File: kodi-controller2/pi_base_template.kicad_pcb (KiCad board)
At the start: 2 copper layers, 109.2 x 62.9 mm, 17 parts, among them P1 Raspberry_Pi_+_Conn, SW1 SW_PUSH_SMALL, SW2 SW_PUSH_SMALL, SW3 SW_PUSH_SMALL, SW4 SW_PUSH_SMALL

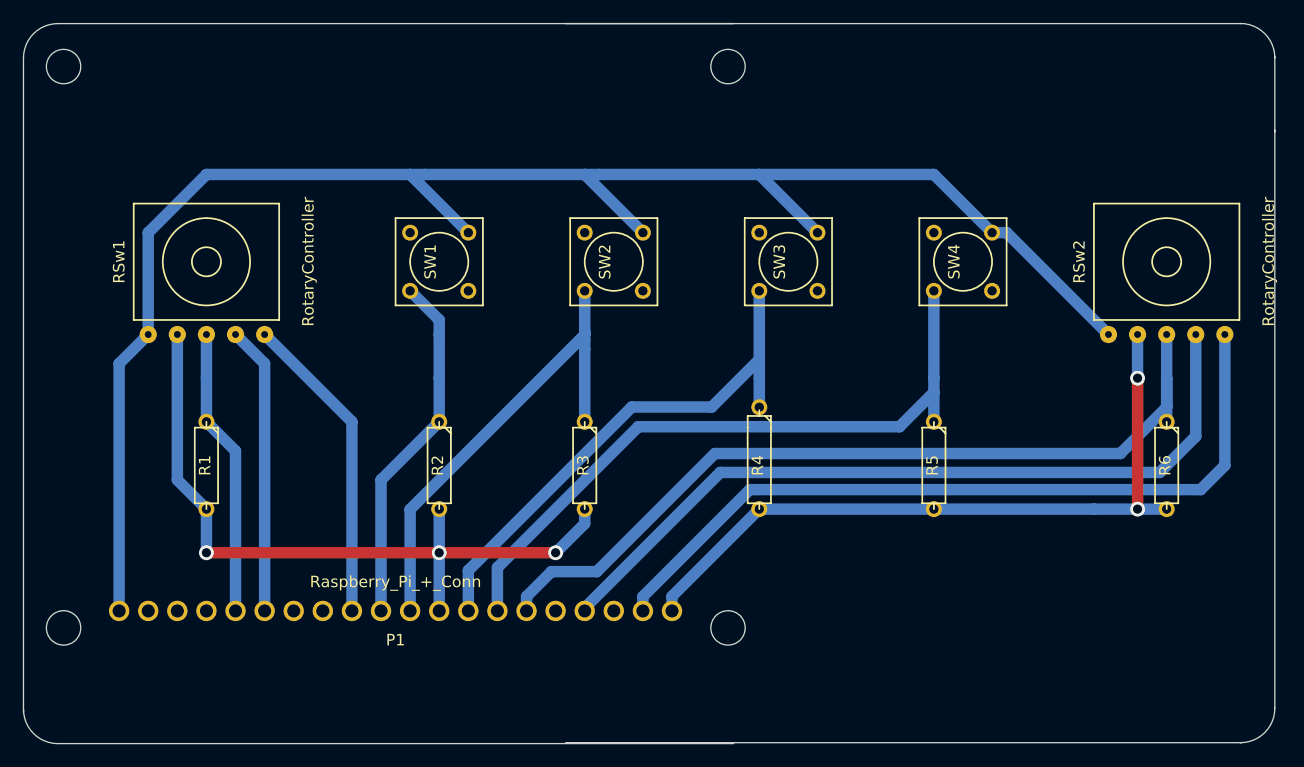
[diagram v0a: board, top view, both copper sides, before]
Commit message: Filled the board once more.
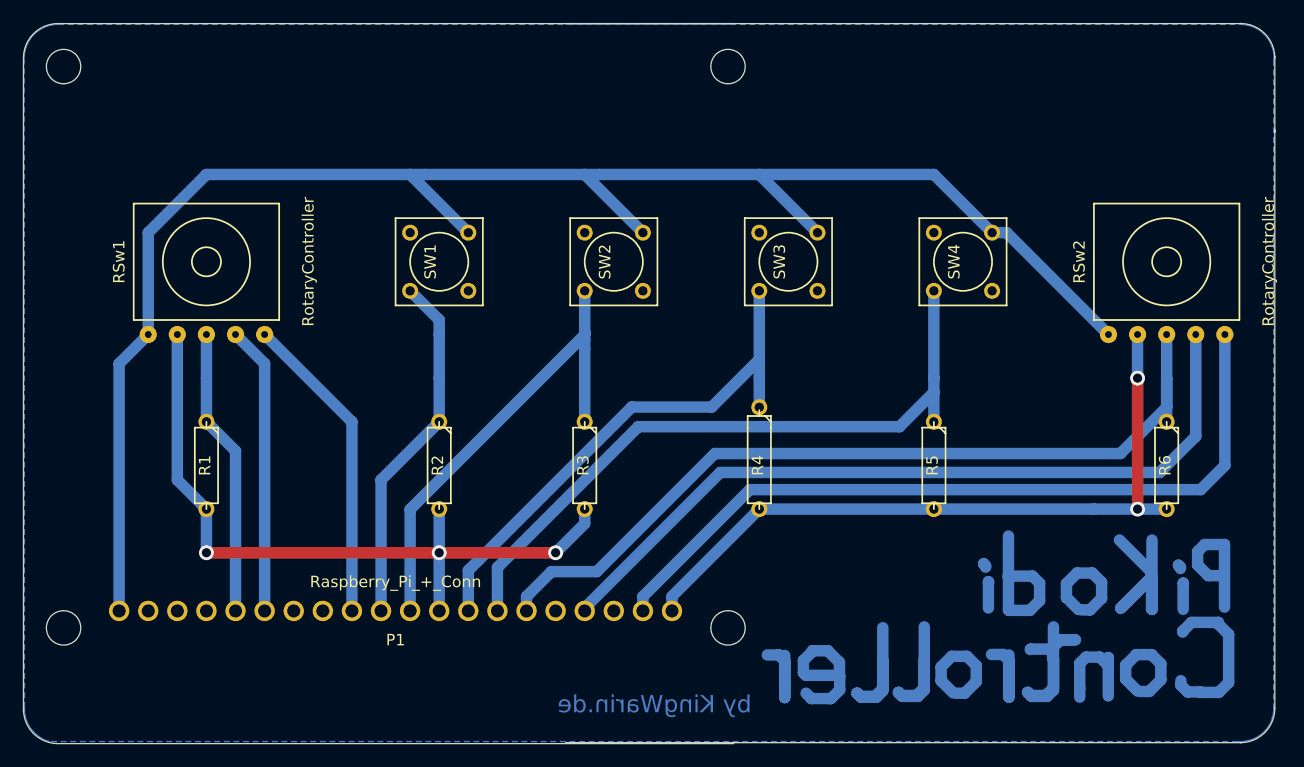
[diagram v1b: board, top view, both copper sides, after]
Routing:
- net (no net): track 0.00 -> 186.0 mm
- added copper zone on B.Cu, net (none)
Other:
- board text added: "by KingWarin.de"
